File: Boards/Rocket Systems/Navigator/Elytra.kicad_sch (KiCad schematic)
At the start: 3 parts, among them U9 SQJA36EP-T1_GE3

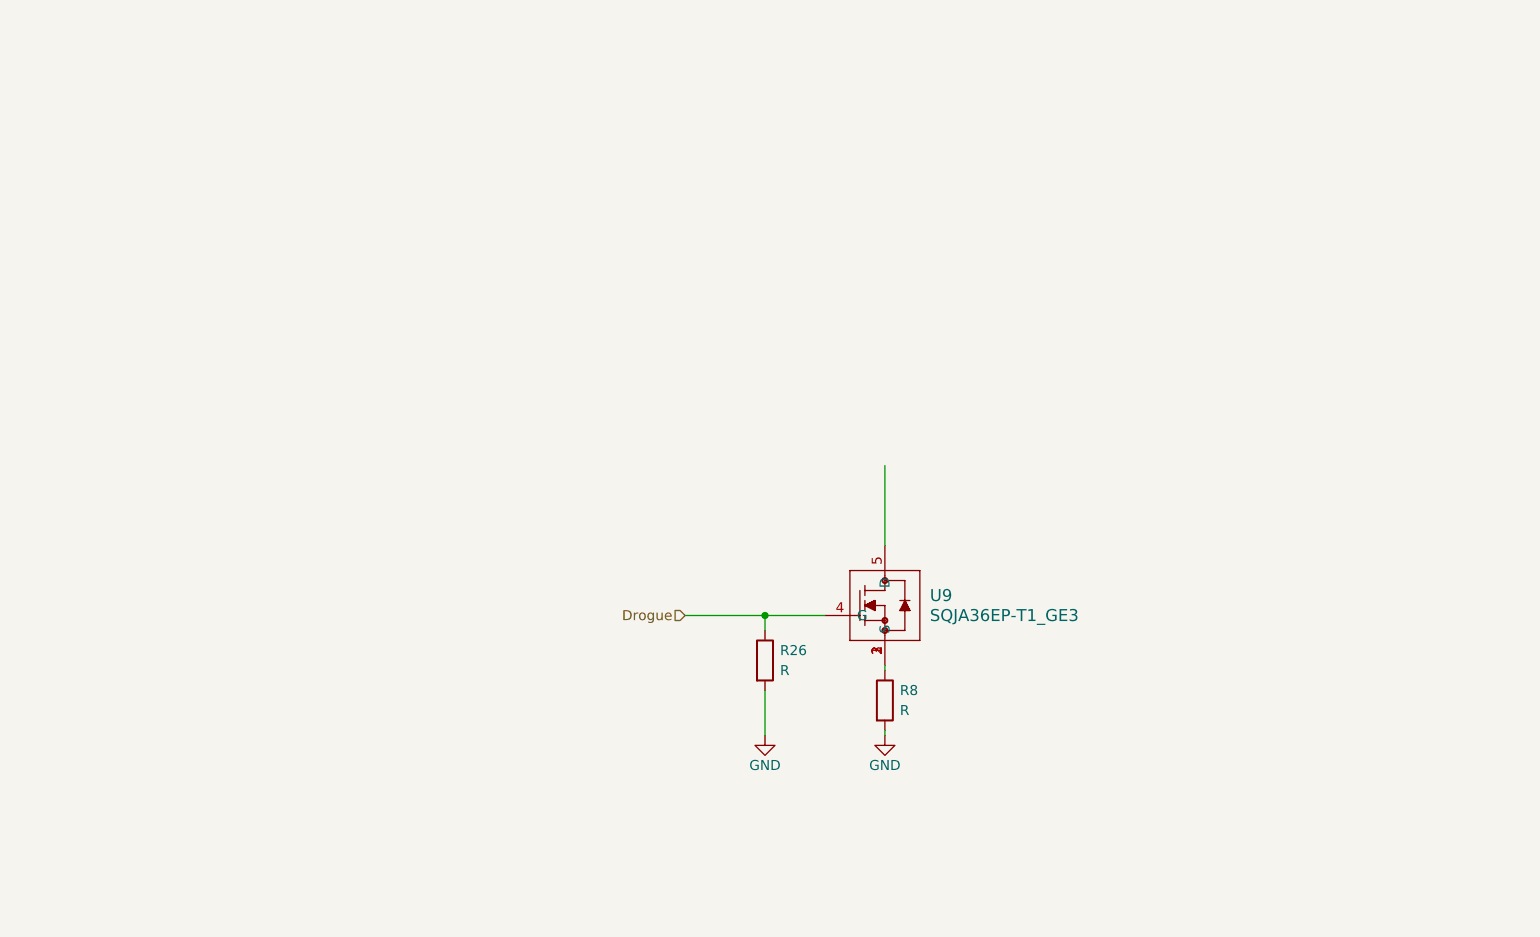
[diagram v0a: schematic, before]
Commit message: HYDRA Update
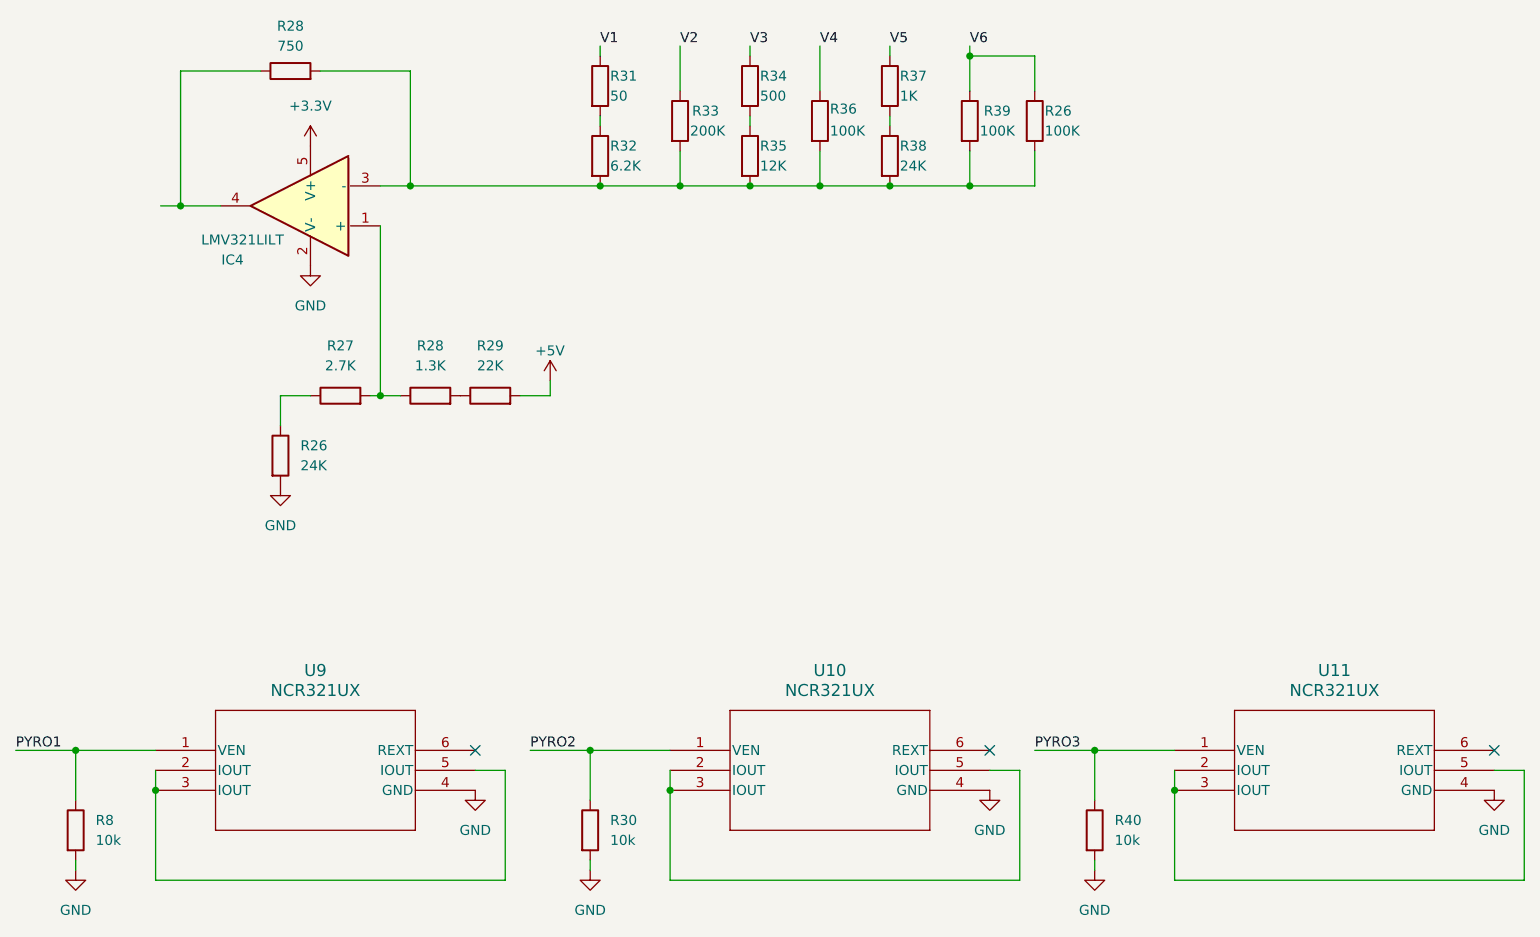
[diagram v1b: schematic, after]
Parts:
- removed R26: R, symbol Device:R
- removed U9: SQJA36EP-T1_GE3, PowerPAK_SO-8L_3_VIS, symbol SQJA36EP-T1-GE3:SQJA36EP-T1_GE3
- added IC4: LMV321LILT, SOT95P280X145-5N, symbol LMV321LILT:LMV321LILT
- added R26: 24K, RES_0402, symbol Device:R
- added R26, R36, R39: 100K, RES_0603, symbol Device:R
- added R27: 2.7K, RES_0402, symbol Device:R
- added R28: 750, RES_0805, symbol Device:R
- added R28: 1.3K, RES_0402, symbol Device:R
- added R29: 22K, RES_0402, symbol Device:R
- added R30, R40: 10k, RES_0402, symbol Device:R
- added R31: 50, RES_0603, symbol Device:R
- added R32: 6.2K, RES_0603, symbol Device:R
- added R33: 200K, RES_0603, symbol Device:R
- added R34: 500, RES_0603, symbol Device:R
- added R35: 12K, RES_0603, symbol Device:R
- added R37: 1K, RES_0603, symbol Device:R
- added R38: 24K, RES_0603, symbol Device:R
- added U10, U11, U9: NCR321UX, TSOP6_SOT457_NEX, symbol NCR321UX:NCR321UX
- R8: value R -> 10k; footprint (none) -> RES_0402
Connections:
- net GND: now also IC4.2 (V-), R26.2, R30.2, R40.2, U10.4 (GND), U11.4 (GND), U9.4 (GND)
- net PYRO1: now reaches R8.1
- net PYRO1: now also U9.1 (VEN)
- new net: IC4.3 (-), R26.2, R28.2, R32.2, R33.2, R35.2, R36.2, R38.2, R39.2
- new net: R37.2, R38.1
- new net: U10.2 (IOUT), U10.3 (IOUT), U10.5 (IOUT)
- new net: R34.2, R35.1
- new net: R26.1, R27.1
- new net: IC4.1 (+), R27.2, R28.1
- new net: IC4.4, R28.1
- new net: R28.2, R29.1
- new net: R31.2, R32.1
- new net: U9.2 (IOUT), U9.3 (IOUT), U9.5 (IOUT)
- new net: U11.2 (IOUT), U11.3 (IOUT), U11.5 (IOUT)
- new net +3.3V: IC4.5 (V+)
- new net +5V: R29.2
- new net PYRO2: R30.1, U10.1 (VEN)
- new net PYRO3: R40.1, U11.1 (VEN)
- new net V1: R31.1
- new net V2: R33.1
- new net V3: R34.1
- new net V4: R36.1
- new net V5: R37.1
- new net V6: R26.1, R39.1
- no-connect marks 0 -> 3
